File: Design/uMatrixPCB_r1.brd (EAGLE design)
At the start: 39.9 x 39.9 mm, 12 parts

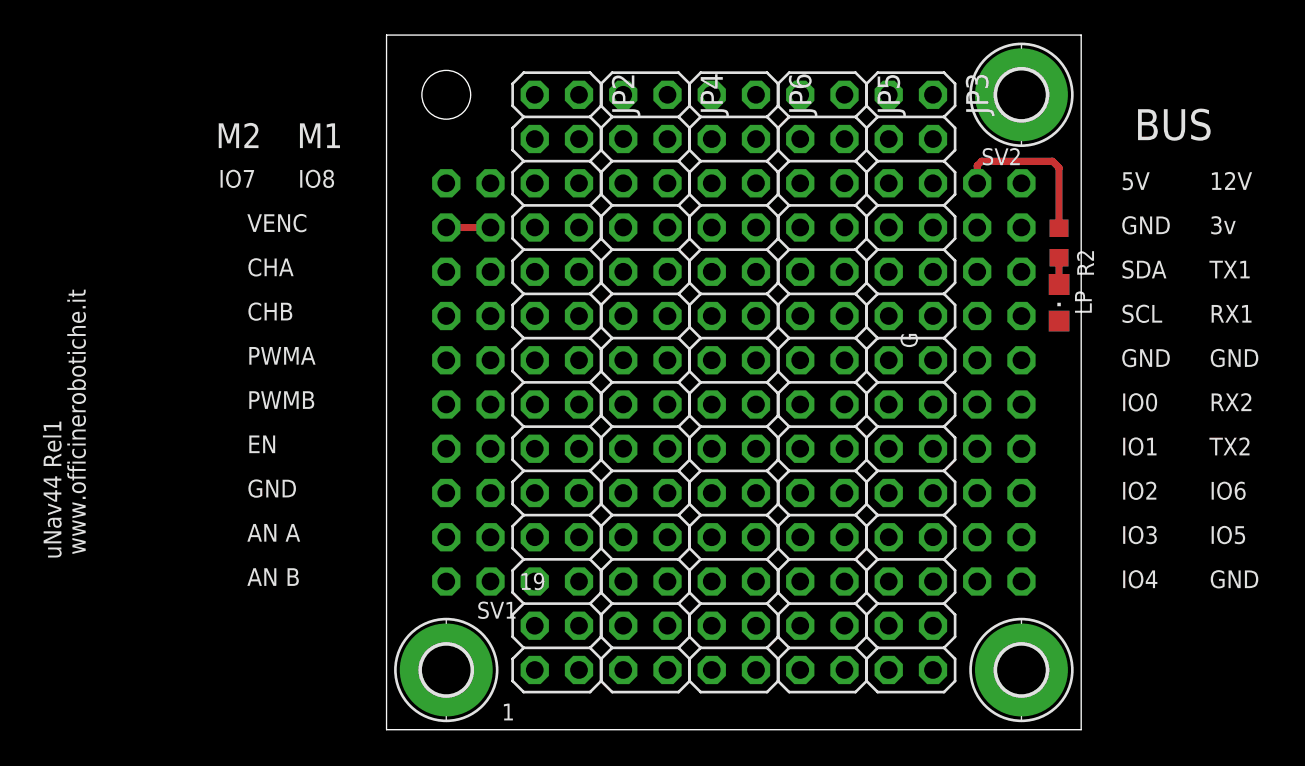
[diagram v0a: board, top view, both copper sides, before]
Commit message: Final Release of Matrix ProtoBoard V1
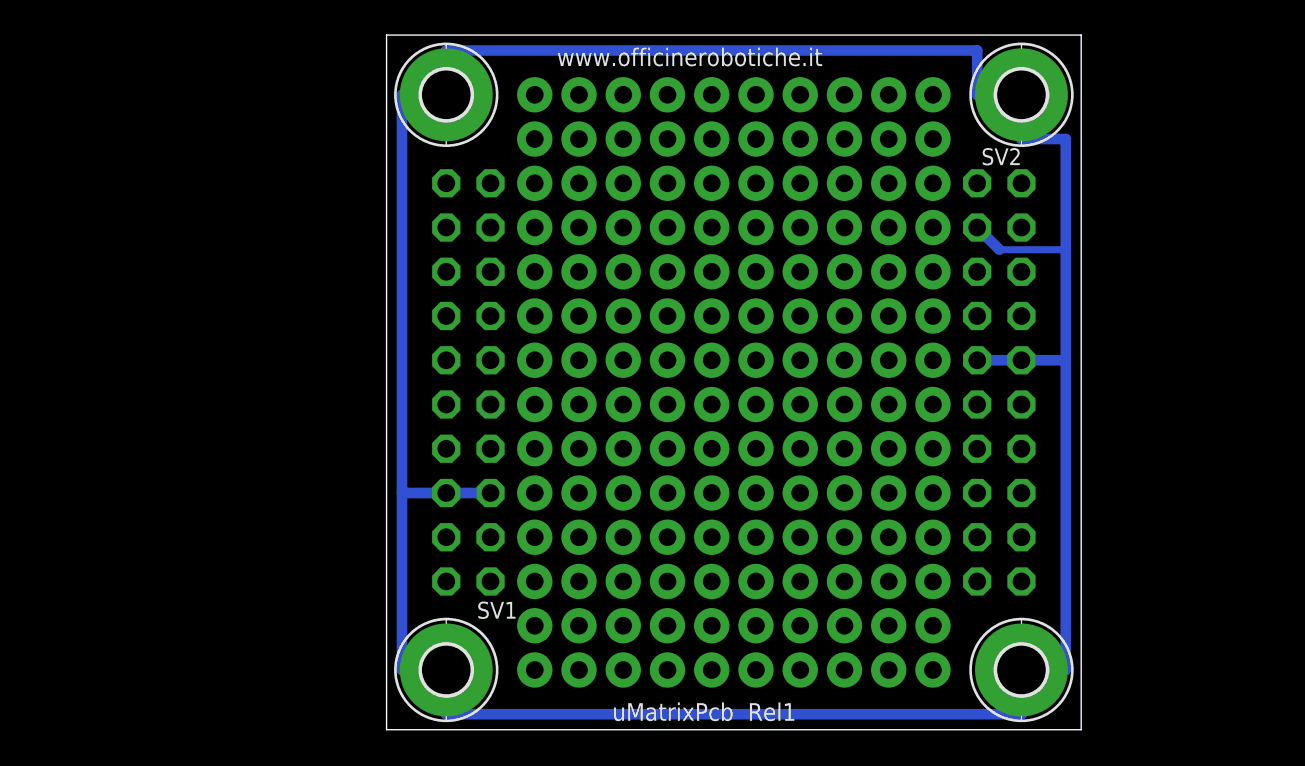
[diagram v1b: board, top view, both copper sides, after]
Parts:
- removed JP2, JP3, JP4, JP5, JP6: (no value), pinhead:2X14
- removed LP: Green, led:CHIPLED_0805
- removed R2: 1K/S 1%, rcl:R0603
- added H4: MOUNT-PAD-ROUND2.8, holes:2,8-PAD
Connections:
- removed net N$5: LP.A, R2.1
- removed net VENC: SV1.3, SV1.4
- new net IO7: SV1.2
- new net IO8: SV1.1
- net +5V: no longer R2.2
- net GND: now also H4.B2,8; no longer LP.C
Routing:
- net GND: track 0.00 -> 168.2 mm
- net +5V: track 9.45 -> 0.00 mm
- net VENC: track 2.54 -> 0.00 mm
- net N$5: track 1.53 -> 0.00 mm, vias 0 -> 1
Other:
- board text added: "uMatrixPcb Rel1"
- board text removed: "+12"
- board text removed: "+3"
- board text removed: "+5"
- board text removed: "+5V"
- board text removed: "1"
- board text removed: "12V"
- board text removed: "19"
- board text removed: "3V"
- board text removed: "3v"
- board text removed: "5V"
- board text removed: "AN A"
- board text removed: "AN B"
- board text removed: "ANA"
- board text removed: "ANB"
- board text removed: "BUS"
- board text removed: "CA"
- board text removed: "CB"
- board text removed: "CHA"
- board text removed: "CHB"
- board text removed: "CZ"
- board text removed: "EN"
- board text removed: "G"
- board text removed: "GND"
- board text removed: "IO0"
- board text removed: "IO1"
- board text removed: "IO2"
- board text removed: "IO3"
- board text removed: "IO4"
- board text removed: "IO5"
- board text removed: "IO6"
- board text removed: "IO7"
- board text removed: "IO8"
- board text removed: "M1"
- board text removed: "M2"
- board text removed: "MCL"
- board text removed: "PA"
- board text removed: "PB"
- board text removed: "PGC"
- board text removed: "PGD"
- board text removed: "PWMA"
- board text removed: "PWMB"
- board text removed: "RX1"
- board text removed: "RX2"
- board text removed: "SCL"
- board text removed: "SDA"
- board text removed: "TX1"
- board text removed: "TX2"
- board text removed: "VENC"
- board text removed: "uNav44 Rel1"
